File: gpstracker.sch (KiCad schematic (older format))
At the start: 52 parts, among them IC1 SIM808, J2 Leds, J3 47553-0001, J4 CONN_COAXIAL, J5 CONN_COAXIAL, J6 Micro_SD_Card, Q1 DMP1045U, SW1 Reset, U1 MCP73832-5-OT, U2 ATMEGA328P-AU, U3 24LC512, U4 MCP1700T-3302E/TT, U5 DS3231SN

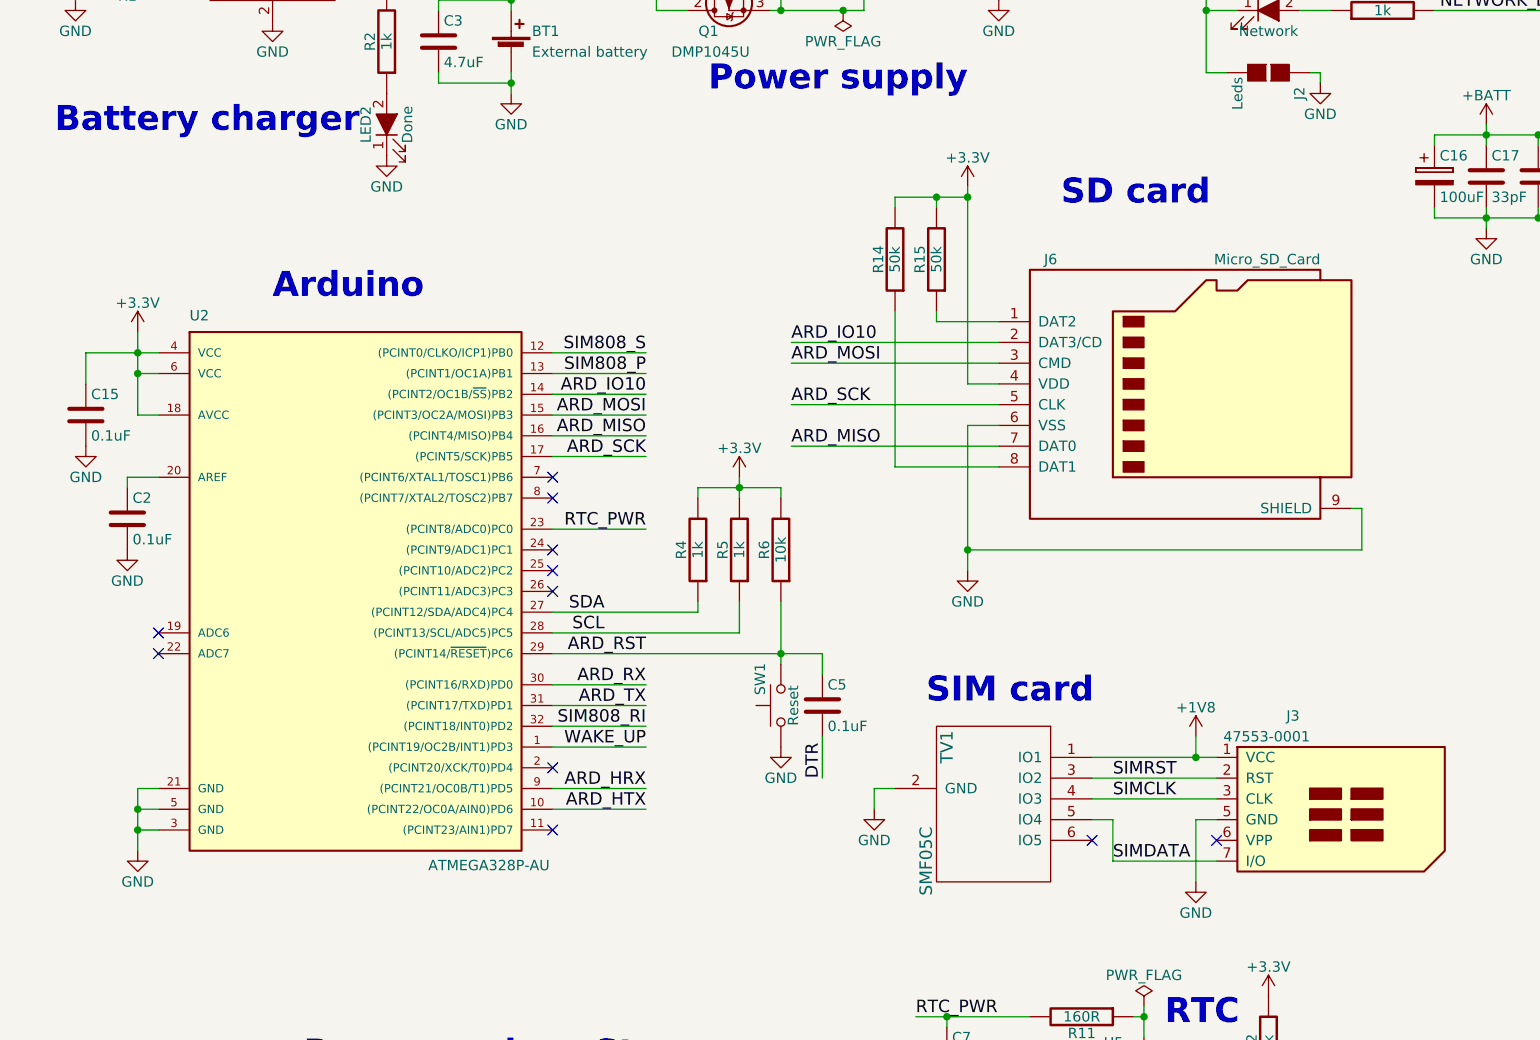
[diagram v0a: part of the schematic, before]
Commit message: More routing
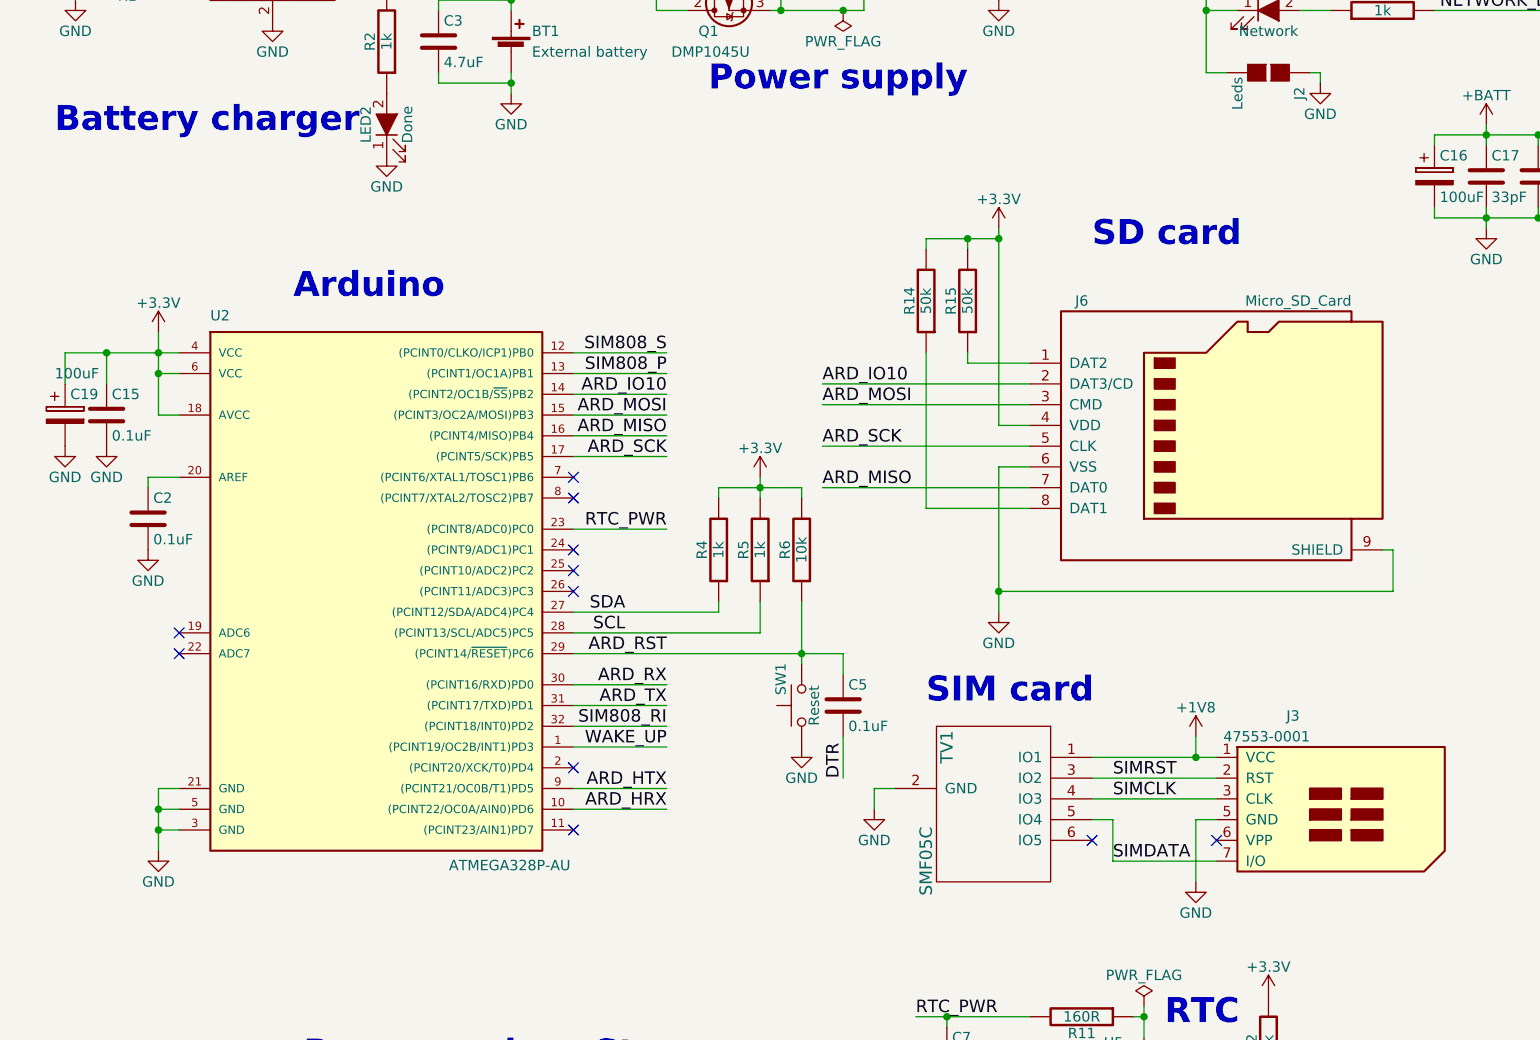
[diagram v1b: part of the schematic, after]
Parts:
- added C19: 100uF, Capacitors_SMD:CP_Elec_6.3x7.7, symbol CP
- C16: footprint Capacitors_Tantalum_SMD:CP_Tantalum_Case-T_EIA-3528-12_Hand -> Capacitors_SMD:CP_Elec_6.3x7.7; Manufacturer (none) -> Panasonic; Manufacturer part number (none) -> EEE-TPC101XAP; Package (none) -> 6.30mm
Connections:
- net +3V3: now also C19.1
- net ARD_HRX: now also U2.10 ((PCINT22/OC0A/AIN0)PD6); no longer U2.9 ((PCINT21/OC0B/T1)PD5)
- net ARD_HTX: now also U2.9 ((PCINT21/OC0B/T1)PD5); no longer U2.10 ((PCINT22/OC0A/AIN0)PD6)
- net GND: now also C19.2
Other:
- moved on the sheet: C15, C2, C5, J6, R14, R15, R4, R5, R6, SW1, U2

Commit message: Redo - Arduino, Sim & power supply
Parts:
- Q1: footprint TO_SOT_Packages_SMD:TO-252-2 -> TO_SOT_Packages_SMD:SOT-23_Handsoldering
- U1: footprint TO_SOT_Packages_SMD:SOT-23-5 -> TO_SOT_Packages_SMD:SOT-23-5_HandSoldering
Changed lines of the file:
@@
 F 0 "U1" H 1300 1550 50  0000 L CNN
 F 1 "MCP73832-5-OT" H 1650 1550 50  0000 L CNN
-F 2 "TO_SOT_Packages_SMD:SOT-23-5" H 1650 1050 50  0001 L CIN
+F 2 "TO_SOT_Packages_SMD:SOT-23-5_HandSoldering" H 1650 1050 50  0001 L CIN
 F 3 "" H 1450 1250 50  0001 C CNN
 	1    1600 1300
@@
 F 0 "Q1" V 4000 1500 50  0000 L CNN
 F 1 "DMP1045U" V 4100 1350 50  0000 L CNN
-F 2 "TO_SOT_Packages_SMD:TO-252-2" H 4000 1550 50  0001 C CNN
+F 2 "TO_SOT_Packages_SMD:SOT-23_Handsoldering" H 4000 1550 50  0001 C CNN
 F 3 "" H 3800 1450 50  0001 C CNN
 	1    3800 1450
